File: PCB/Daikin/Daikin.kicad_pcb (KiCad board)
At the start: 2 copper layers, 13.2 x 19.5 mm, 19 parts, among them J1 1x4, J2 Prog, Q3 PMF250XNEX, U1 ESP32-PICO-MINI-02, U2 LMR16006XDDCR

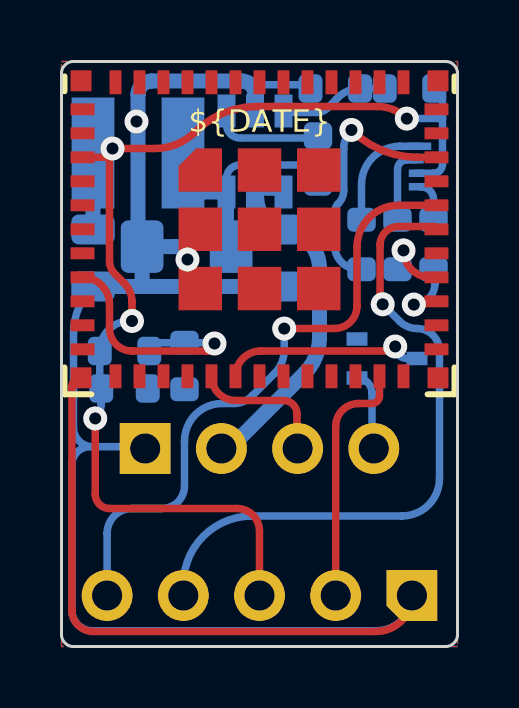
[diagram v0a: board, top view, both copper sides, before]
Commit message: Tidy
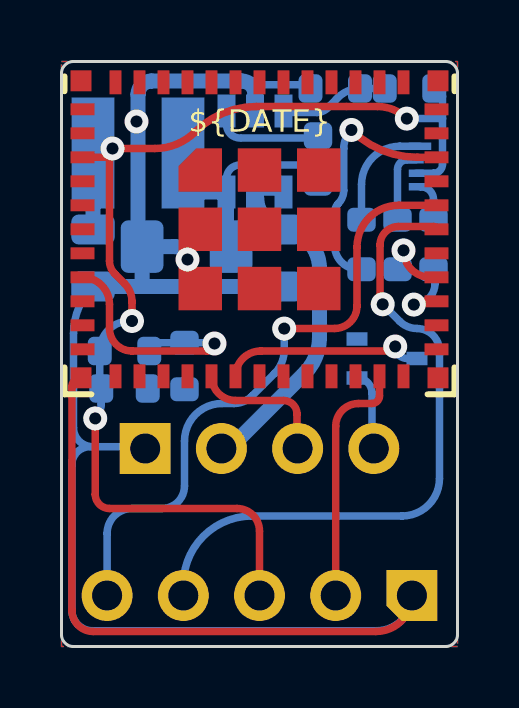
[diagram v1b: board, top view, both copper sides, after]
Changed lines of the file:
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@@
       (options (clearance outline) (anchor rect))
       (primitives
-    (gr_arc (start 0.001745 0.000002) (mid 0.707106 0.292893) (end 0.999998 0.998254) (width 0.5))
+    (gr_arc (start 0.001745 0.000002) (mid 0.706489 0.292277) (end 0.999993 0.996509) (width 0.5))
       ))
     (pad "6" smd rect (at 0.95 -1.35 90) (size 1.1 0.6) (layers "B.Cu" "B.Paste" "B.Mask")

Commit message: Tidy
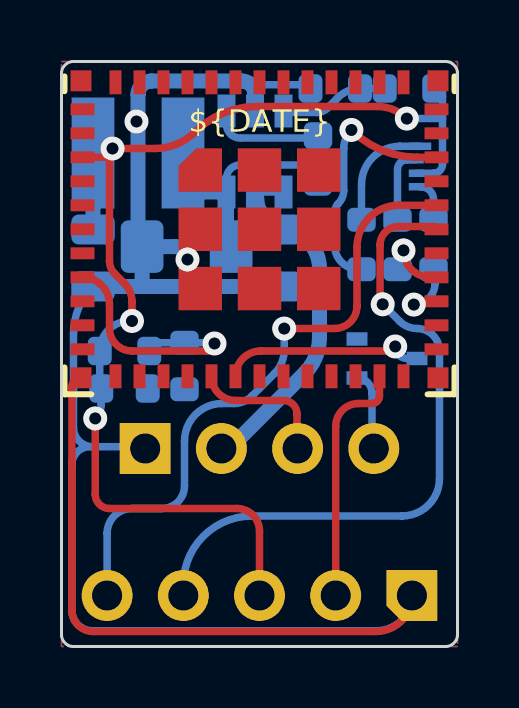
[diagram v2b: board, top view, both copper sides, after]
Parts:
- U2: value LMR16006XDDCR -> LMR16006YDDCR
